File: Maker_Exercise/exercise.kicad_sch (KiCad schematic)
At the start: 35 parts, among them J1 USB_C_Receptacle_USB2.0_16P, J2 Conn_01x02, J3 Conn_ST_STDC14, J4 Conn_01x04, U1 USBLC6-2SC6, U2 STM32G431CBUx

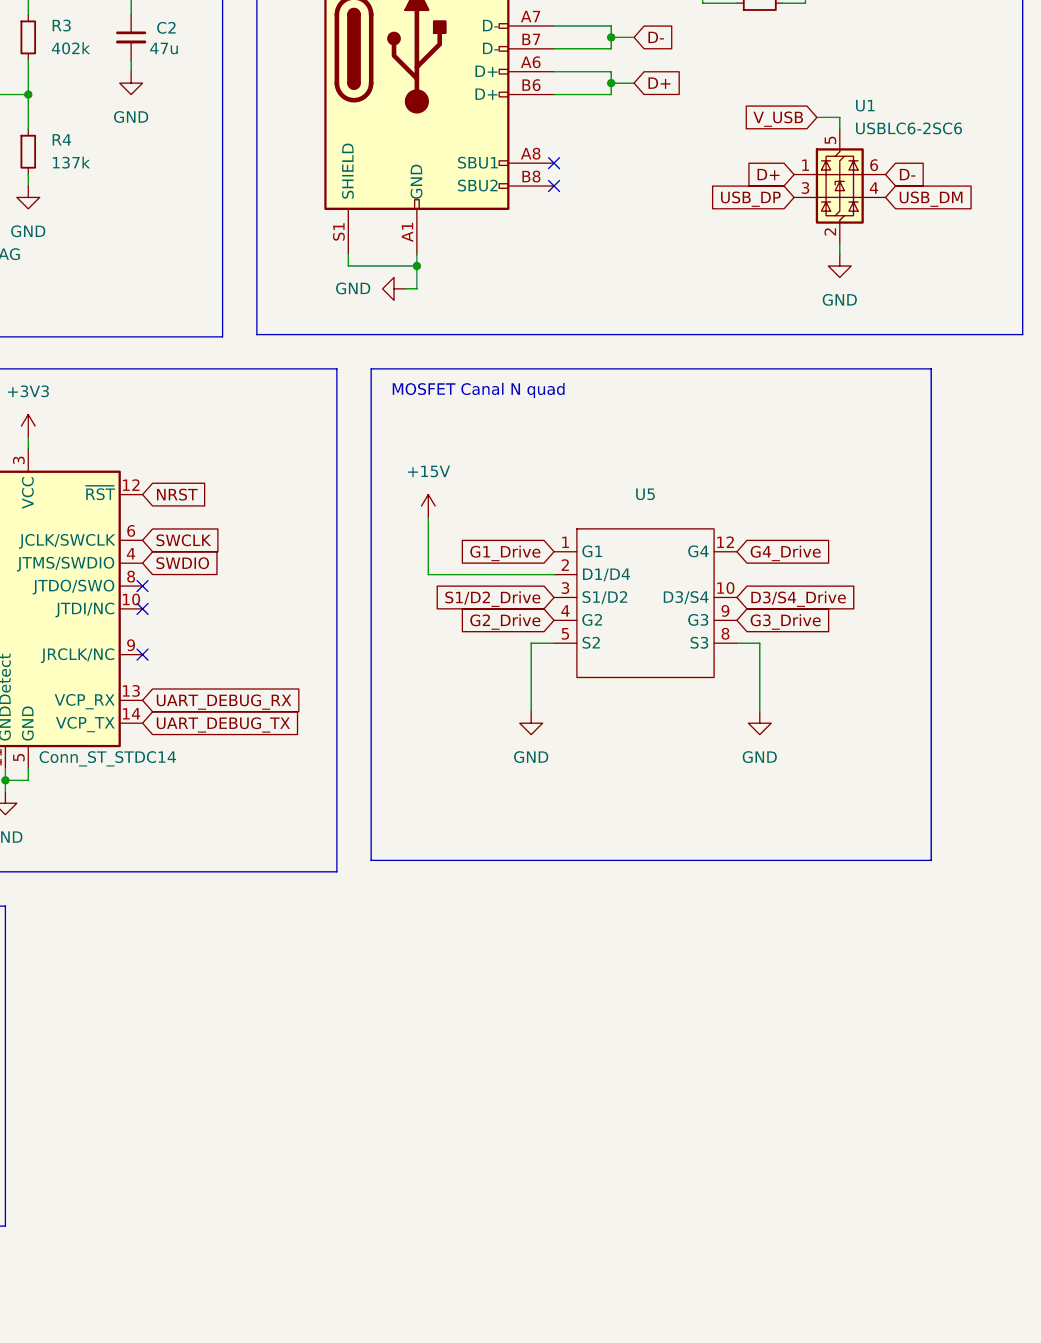
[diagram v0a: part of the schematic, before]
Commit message: finalized PCB and routing
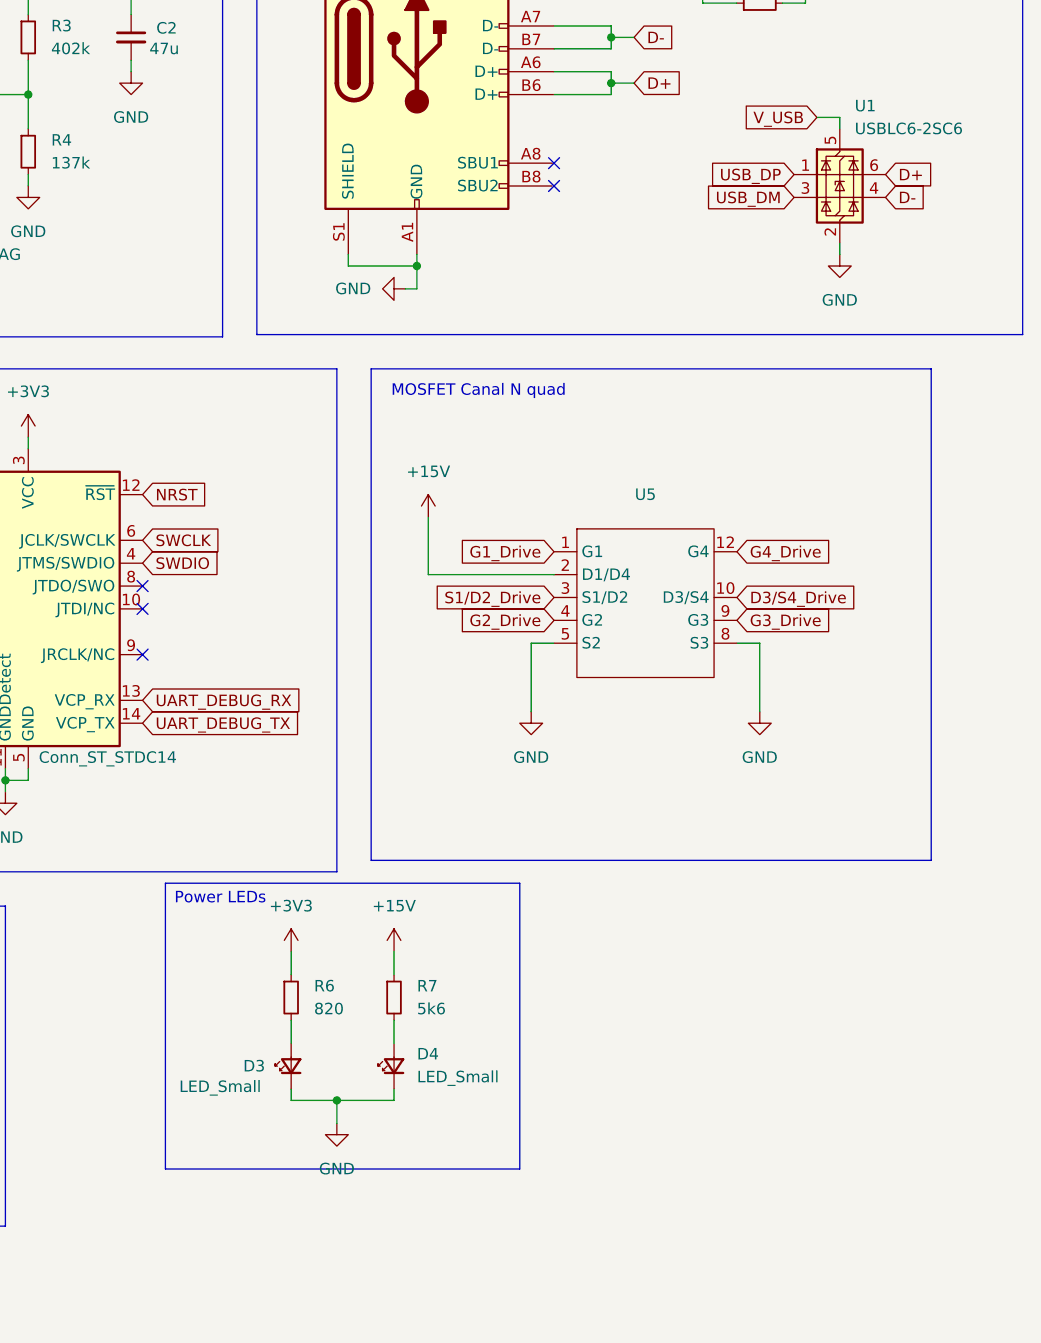
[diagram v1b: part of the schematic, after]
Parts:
- added D3, D4: LED_Small, LED_SMD:LED_0603_1608Metric_Pad1.05x0.95mm_HandSolder, symbol Device:LED_Small
- added R6: 820, Resistor_SMD:R_0402_1005Metric_Pad0.72x0.64mm_HandSolder, symbol Device:R_Small
- added R7: 5k6, Resistor_SMD:R_0402_1005Metric_Pad0.72x0.64mm_HandSolder, symbol Device:R_Small
- C1, C10, C11, C12, C13, C14, C2, C3, C4, C5, C6, C7, C8, C9: footprint Capacitor_SMD:C_0603_1608Metric_Pad1.08x0.95mm_HandSolder -> Capacitor_SMD:C_0402_1005Metric_Pad0.74x0.62mm_HandSolder
- R1, R2, R3, R4, R5: footprint Resistor_SMD:R_0603_1608Metric_Pad0.98x0.95mm_HandSolder -> Resistor_SMD:R_0402_1005Metric_Pad0.72x0.64mm_HandSolder
- U2: MPN (none) -> STM32G431CBU6
- U4: MPN (none) -> 171013801
- U5: MPN (none) -> FDMQ86530L
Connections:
- net +15V: now also R7.1
- net +3V3: now also R6.1
- net D+: now also U1.6 (I/O1); no longer U1.1 (I/O1)
- net D-: now also U1.4 (I/O2); no longer U1.6 (I/O1)
- net GND: now also D3.1 (K), D4.1 (K)
- net USB_DM: now also U1.3 (I/O2); no longer U1.4 (I/O2)
- net USB_DP: now also U1.1 (I/O1); no longer U1.3 (I/O2)
- new net: D3.2 (A), R6.2
- new net: D4.2 (A), R7.2
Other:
- note added: "Power LEDs"
